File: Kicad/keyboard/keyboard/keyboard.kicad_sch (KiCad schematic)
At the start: 89 parts, among them J1 Conn_01x05_Pin, J2 Conn_01x08_Pin, SW1 ESC, SW10 Q, SW11 S, SW12 G, SW13 Y, SW14 J, SW15 K, SW16 P, SW17 Shift, SW18 A, SW19 D, SW2 W, SW20 V, SW21 H, SW22 M, SW23 L, SW24 BackSpace, SW25 Menu, SW26 Z, SW27 F, SW28 B, SW29 N, SW3 E, SW30 ||, SW31 ., SW32 Enter, SW33 Ctrl, SW34 X, SW35 C, SW36 Space, SW37 Up, SW38 Left, SW39 Down, SW4 R, SW40 Right, SW5 T, SW6 U, SW7 I, SW8 O, SW9 Alt

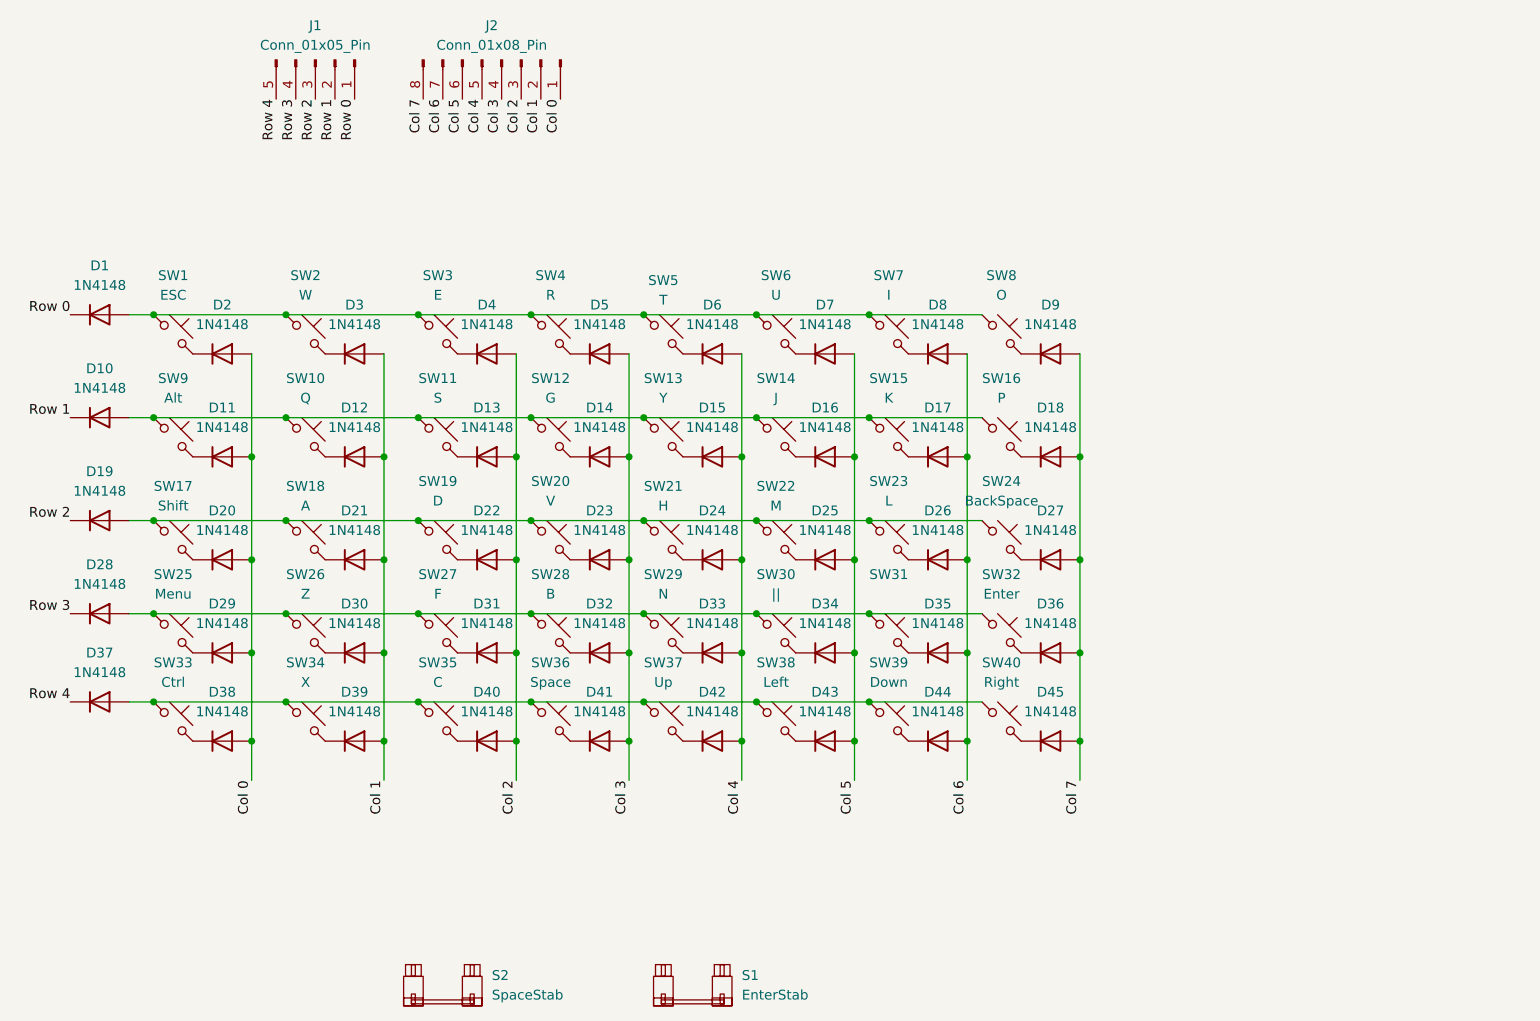
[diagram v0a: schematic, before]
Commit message: v2a update
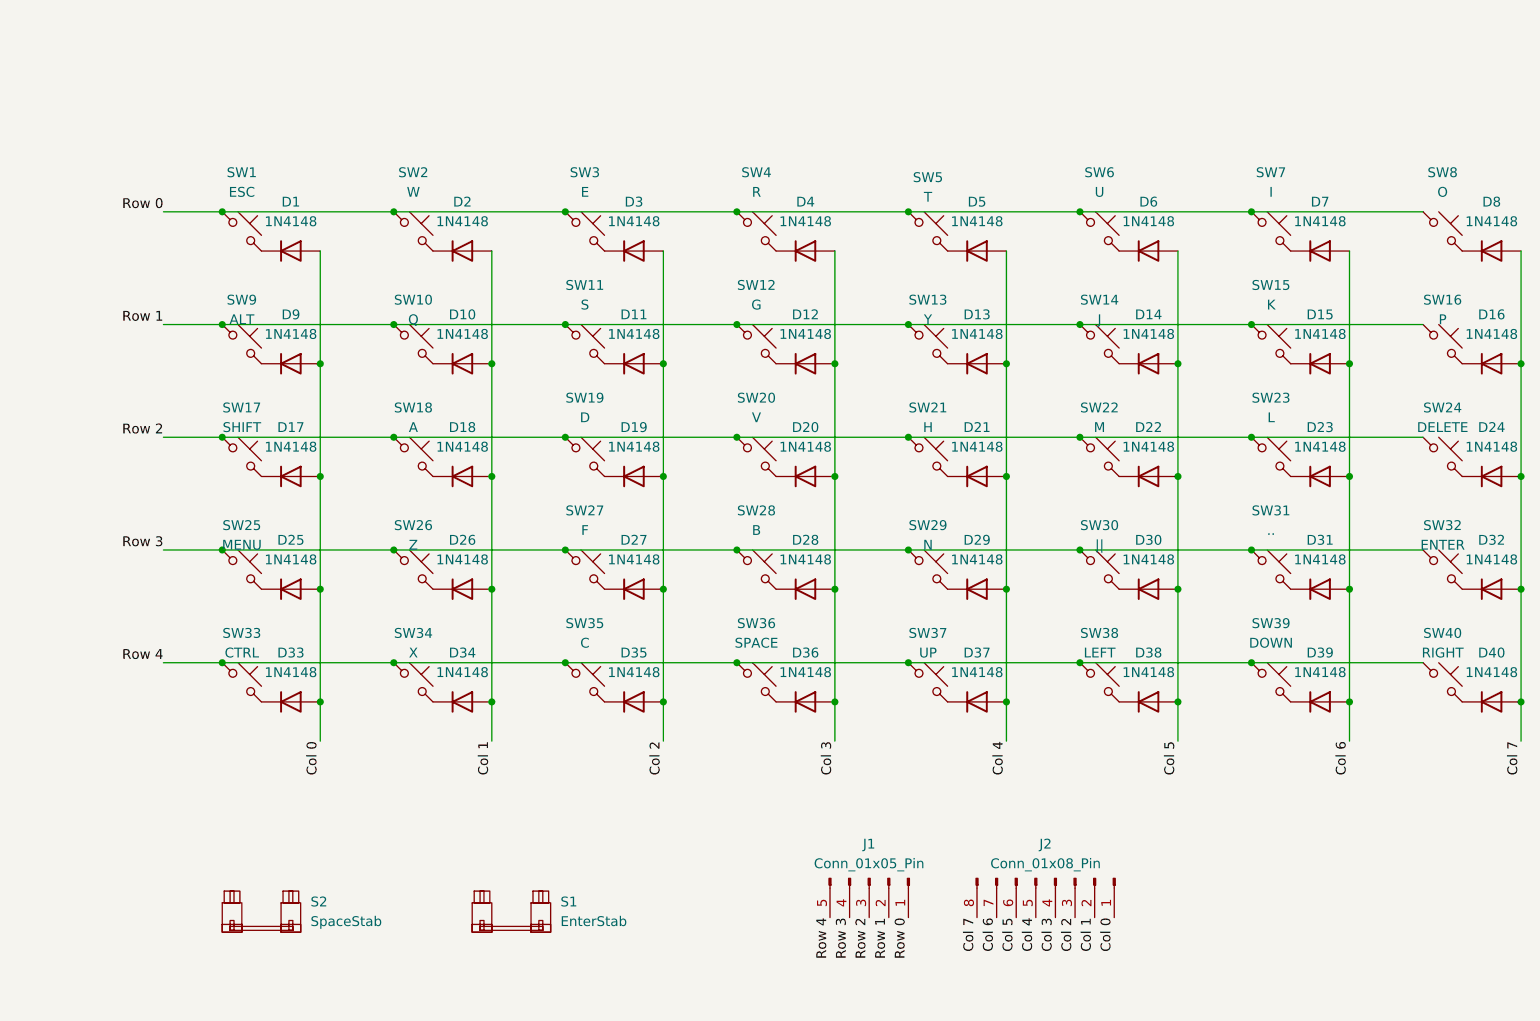
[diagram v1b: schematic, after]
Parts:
- removed D41, D42, D43, D44, D45: 1N4148, Diode_THT:D_DO-35_SOD27_P7.62mm_Horizontal, symbol Diode:1N4148
- S1: footprint PCM_marbastlib-mx:STAB_MX_P_2u -> KS27_PCB_STAB:ks27_2u_pcb_cherry_plate_stab
- S2: footprint PCM_marbastlib-mx:STAB_MX_P_6.25u -> KS27_PCB_STAB:ks26_6.25u_pcb_cherry_plate
- SW1, SW10, SW11, SW12, SW13, SW14, SW15, SW16, SW18, SW19, SW2, SW20, SW21, SW22, SW23, SW26, SW27, SW28, SW29, SW3, SW34, SW35, SW4, SW5, SW6, SW7, SW8: footprint keyswitches.pretty-2.1:SW_PG1350_MX_Hybrid -> SMAL:SW_Redragon_LowProfile_PCB_1.00u
- SW17: value Shift -> SHIFT; footprint keyswitches.pretty-2.1:SW_PG1350_MX_Hybrid -> SMAL:SW_Redragon_LowProfile_PCB_1.75u
- SW24: value BackSpace -> DELETE; footprint keyswitches.pretty-2.1:SW_PG1350_MX_Hybrid -> SMAL:SW_Redragon_LowProfile_PCB_1.25u
- SW25: value Menu -> MENU; footprint keyswitches.pretty-2.1:SW_PG1350_MX_Hybrid -> SMAL:SW_Redragon_LowProfile_PCB_1.75u
- SW30: footprint keyswitches.pretty-2.1:SW_PG1350_MX_Hybrid -> SMAL:SW_Redragon_LowProfile_PCB_1.50u
- SW31: value . -> ..; footprint keyswitches.pretty-2.1:SW_PG1350_MX_Hybrid -> SMAL:SW_Redragon_LowProfile_PCB_1.00u
- SW32: value Enter -> ENTER; footprint keyswitches.pretty-2.1:SW_PG1350_MX_Hybrid -> SMAL:SW_Redragon_LowProfile_PCB_2.00u
- SW33: value Ctrl -> CTRL; footprint keyswitches.pretty-2.1:SW_PG1350_MX_Hybrid -> SMAL:SW_Redragon_LowProfile_PCB_1.25u
- SW36: value Space -> SPACE; footprint keyswitches.pretty-2.1:SW_PG1350_MX_Hybrid -> SMAL:SW_Redragon_LowProfile_PCB_6.25u
- SW37: value Up -> UP; footprint keyswitches.pretty-2.1:SW_PG1350_MX_Hybrid -> SMAL:SW_Redragon_LowProfile_PCB_1.00u
- SW38: value Left -> LEFT; footprint keyswitches.pretty-2.1:SW_PG1350_MX_Hybrid -> SMAL:SW_Redragon_LowProfile_PCB_1.00u
- SW39: value Down -> DOWN; footprint keyswitches.pretty-2.1:SW_PG1350_MX_Hybrid -> SMAL:SW_Redragon_LowProfile_PCB_1.00u
- SW40: value Right -> RIGHT; footprint keyswitches.pretty-2.1:SW_PG1350_MX_Hybrid -> SMAL:SW_Redragon_LowProfile_PCB_1.00u
- SW9: value Alt -> ALT; footprint keyswitches.pretty-2.1:SW_PG1350_MX_Hybrid -> SMAL:SW_Redragon_LowProfile_PCB_1.25u
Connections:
- net Col 0: now also D1.2 (A), D17.2 (A), D25.2 (A), D33.2 (A), D9.2 (A); no longer D11.2 (A), D2.2 (A), D20.2 (A), D29.2 (A), D38.2 (A)
- net Col 1: now also D10.2 (A), D18.2 (A), D2.2 (A), D26.2 (A), D34.2 (A); no longer D12.2 (A), D21.2 (A), D3.2 (A), D30.2 (A), D39.2 (A)
- net Col 2: now also D11.2 (A), D19.2 (A), D27.2 (A), D3.2 (A), D35.2 (A); no longer D13.2 (A), D22.2 (A), D31.2 (A), D4.2 (A), D40.2 (A)
- net Col 3: now also D12.2 (A), D20.2 (A), D28.2 (A), D36.2 (A), D4.2 (A); no longer D14.2 (A), D23.2 (A), D32.2 (A), D5.2 (A)
- net Col 4: now also D13.2 (A), D21.2 (A), D29.2 (A), D37.2 (A), D5.2 (A); no longer D15.2 (A), D24.2 (A), D33.2 (A), D6.2 (A)
- net Col 5: now also D14.2 (A), D22.2 (A), D30.2 (A), D38.2 (A), D6.2 (A); no longer D16.2 (A), D25.2 (A), D34.2 (A), D7.2 (A)
- net Col 6: now also D15.2 (A), D23.2 (A), D31.2 (A), D39.2 (A), D7.2 (A); no longer D17.2 (A), D26.2 (A), D35.2 (A), D8.2 (A)
- net Col 7: now also D16.2 (A), D24.2 (A), D32.2 (A), D40.2 (A), D8.2 (A); no longer D18.2 (A), D27.2 (A), D36.2 (A), D9.2 (A)
- net Row 0: now also SW1.1, SW2.1, SW3.1, SW4.1, SW5.1, SW6.1, SW7.1, SW8.1; no longer D1.1 (K)
- net Row 1: now also SW10.1, SW11.1, SW12.1, SW13.1, SW14.1, SW15.1, SW16.1, SW9.1; no longer D10.1 (K)
- net Row 2: now also SW17.1, SW18.1, SW19.1, SW20.1, SW21.1, SW22.1, SW23.1, SW24.1; no longer D19.1 (K)
- net Row 3: now also SW25.1, SW26.1, SW27.1, SW28.1, SW29.1, SW30.1, SW31.1, SW32.1; no longer D28.1 (K)
- net Row 4: now also SW33.1, SW34.1, SW35.1, SW36.1, SW37.1, SW38.1, SW39.1, SW40.1; no longer D37.1 (K)
- net at SW19.2: now also D19.1 (K); no longer D22.1 (K)
- net at D20.1 (K): now also SW20.2; no longer SW17.2
- net at SW35.2: now also D35.1 (K); no longer D40.1 (K)
- net at D3.1 (K): now also SW3.2; no longer SW2.2
- net at SW40.2: now also D40.1 (K)
- net at SW39.2: now also D39.1 (K)
- net at SW23.2: now also D23.1 (K); no longer D26.1 (K)
- net at SW28.2: now also D28.1 (K); no longer D32.1 (K)
- net at SW37.2: now also D37.1 (K)
- net at D31.1 (K): now also SW31.2; no longer SW27.2
- net at SW32.2: now also D32.1 (K); no longer D36.1 (K)
- net at SW34.2: now also D34.1 (K); no longer D39.1 (K)
- net at SW5.2: now also D5.1 (K); no longer D6.1 (K)
- net at SW13.2: now also D13.1 (K); no longer D15.1 (K)
- net at SW9.2: now also D9.1 (K); no longer D11.1 (K)
- net at SW4.2: now also D4.1 (K); no longer D5.1 (K)
- net at SW21.2: now also D21.1 (K); no longer D24.1 (K)
- net at D8.1 (K): now also SW8.2; no longer SW7.2
- net at SW12.2: now also D12.1 (K); no longer D14.1 (K)
- net at SW10.2: now also D10.1 (K); no longer D12.1 (K)
- net at SW24.2: now also D24.1 (K); no longer D27.1 (K)
- net at SW36.2: now also D36.1 (K)
- net at SW16.2: now also D16.1 (K); no longer D18.1 (K)
- net at SW33.2: now also D33.1 (K); no longer D38.1 (K)
- net at SW22.2: now also D22.1 (K); no longer D25.1 (K)
- net at D7.1 (K): now also SW7.2; no longer SW6.2
- net at D29.1 (K): now also SW29.2; no longer SW25.2
- net at SW30.2: now also D30.1 (K); no longer D34.1 (K)
- net at SW38.2: now also D38.1 (K)
- net at SW11.2: now also D11.1 (K); no longer D13.1 (K)
- net at SW14.2: now also D14.1 (K); no longer D16.1 (K)
- net at SW18.2: now also D18.1 (K); no longer D21.1 (K)
- net at SW1.2: now also D1.1 (K); no longer D2.1 (K)
- net at D17.1 (K): now also SW17.2; no longer SW15.2
- net at SW26.2: now also D26.1 (K); no longer D30.1 (K)
- new net: D2.1 (K), SW2.2
- new net: D25.1 (K), SW25.2
- new net: D15.1 (K), SW15.2
- new net: D27.1 (K), SW27.2
- new net: D6.1 (K), SW6.2
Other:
- moved on the sheet: J1, J2, S1, S2
